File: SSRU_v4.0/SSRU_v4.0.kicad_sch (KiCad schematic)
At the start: 69 parts, among them J2 Conn_01x24, J4 AVR-ISP-6, SW1 SW_Push, U1 SGM722, U10 TJA1051T, U2 ATmega328P-A, U3 SGM722, U4 LM2576S-5, U6 MCP2515-xST, U69 SGM722, Y1 16MHz, Y4 20MHz

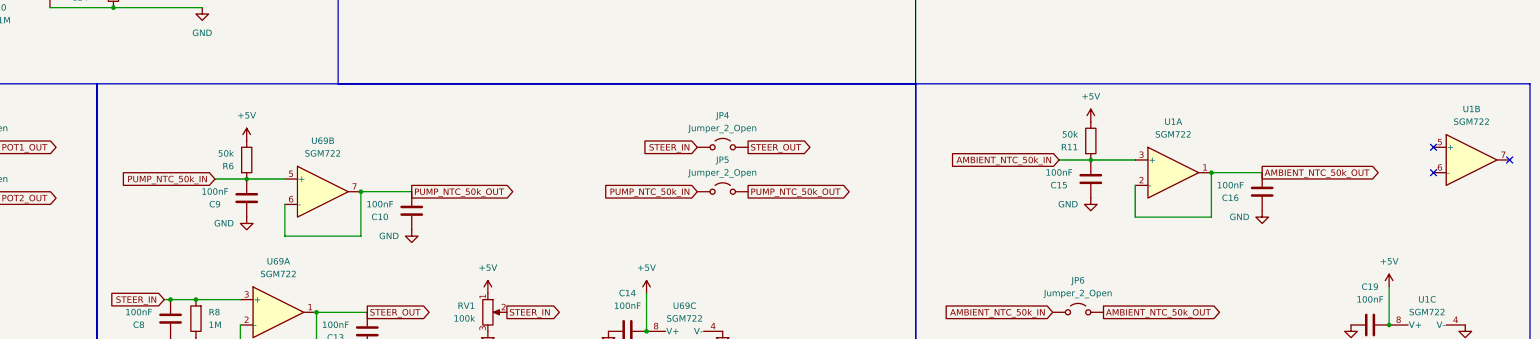
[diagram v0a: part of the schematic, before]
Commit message: helo
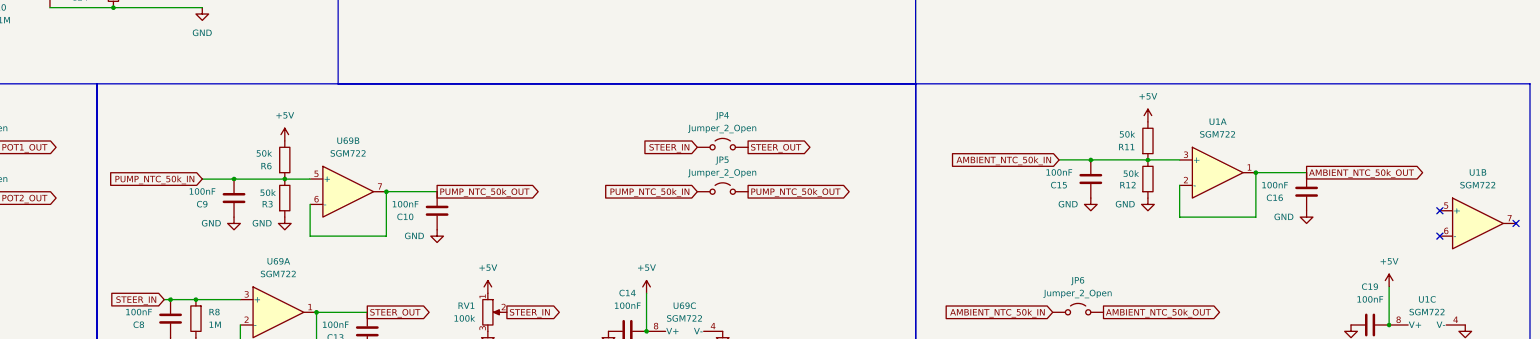
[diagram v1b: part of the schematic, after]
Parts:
- added R12, R3: 50k, RMC_Resistor:R_0805_2012Metric_Pad1.20x1.40mm_HandSolder_L, symbol Device:R
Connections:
- net AMBIENT_NTC_50k_IN: now also R12.1
- net GND: now also R12.2, R3.2
- net PUMP_NTC_50k_IN: now also R3.1
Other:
- moved on the sheet: C10, C16, C9, R11, R6, U1A, U1B, U69B
